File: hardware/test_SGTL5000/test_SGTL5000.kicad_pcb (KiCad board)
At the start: 2 copper layers, 68 x 68 mm, 70 parts, among them J201 SWD, J301 LINEIN_R, J302 LINEIN_L, J303 MIC, J304 LINEOUT_L, J305 LINEOUT_R, J401 USB_C_Receptacle_USB2.0, SW201 RST, U201 STM32G431KBT6, U301 SGTL5000XNLA3, U401 USBLC6-2SC6, U501 BU33SD5WG-TR, U502 BU33SD5WG-TR, U503 BU18SD2MG-MTR, Y201 16MHz

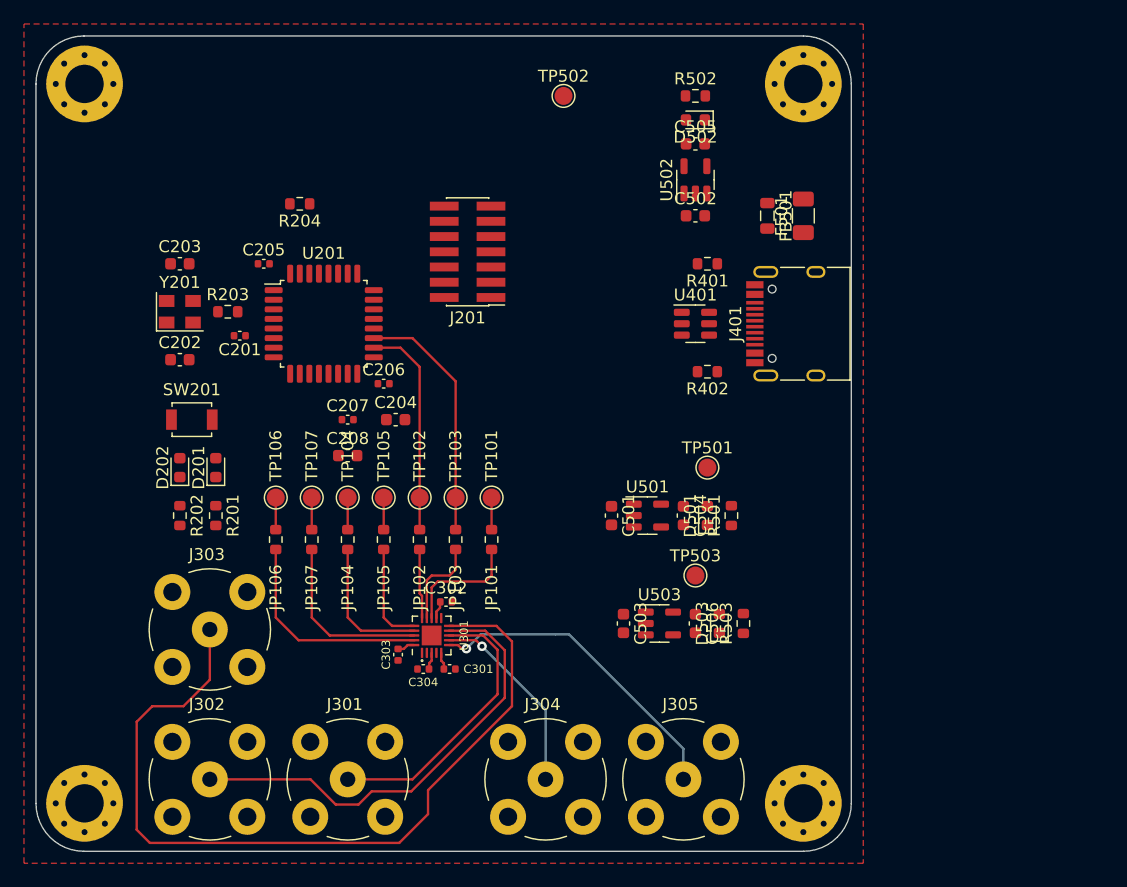
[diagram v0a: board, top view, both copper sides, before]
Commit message: Started routing
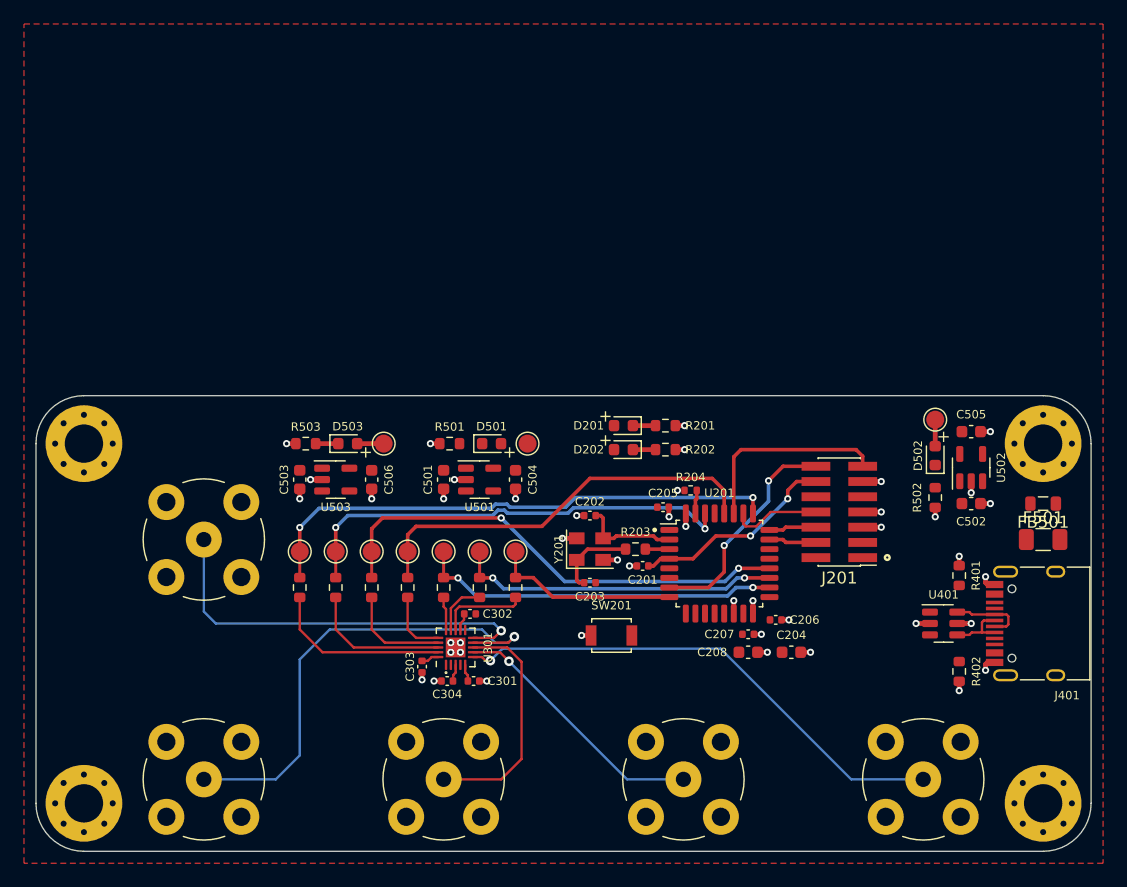
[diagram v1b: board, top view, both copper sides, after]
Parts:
- C202, C203: footprint Capacitor_SMD:C_0603_1608Metric -> Capacitor_SMD:C_0402_1005Metric
- R204: footprint Resistor_SMD:R_0603_1608Metric -> Resistor_SMD:R_0402_1005Metric
- moved C203 43.3 mm to (62.2, 61.6), turned to 180 degrees
- moved TP502 41.1 mm to (91.0, 48.0)
- moved R202 40.9 mm to (68.5, 50.5), turned to 0 degrees
- moved R204 40.4 mm to (70.6, 53.9)
- moved Y201 39.5 mm to (62.2, 58.8)
- moved R503 39.5 mm to (38.5, 50.0), turned to 180 degrees
- moved SW201 39.4 mm to (64.0, 66.0)
- moved R203 39.3 mm to (66.0, 58.8)
- moved R502 39.0 mm to (91.0, 54.5), turned to -90 degrees
- moved C205 39.0 mm to (68.3, 55.3)
- moved C201 38.7 mm to (66.6, 60.2)
- moved U201 38.6 mm to (73.0, 60.0)
- moved C204 38.3 mm to (79.0, 67.4)
- moved R201 38.2 mm to (68.5, 48.5), turned to 0 degrees
- moved C206 38.2 mm to (77.7, 64.7)
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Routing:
- net /STM32/I2C_SCL: track 2.67 -> 44.5 mm, vias 0 -> 2
- net /STM32/I2S_DIN: track 2.67 -> 40.3 mm, vias 0 -> 2
- net /CODEC/MIC: track 69.6 -> 34.1 mm, vias 0 -> 1
- net GND: track 0.00 -> 35.3 mm, vias 0 -> 43
- net /STM32/I2C_SDA: track 2.67 -> 37.9 mm, vias 0 -> 2
- net /STM32/I2S_DOUT: track 2.67 -> 34.3 mm
- net /STM32/VCP_TX: track 0.00 -> 18.7 mm, vias 0 -> 2
- net /STM32/nRST: track 0.00 -> 17.3 mm, vias 0 -> 2
- net /STM32/VCP_RX: track 0.00 -> 16.8 mm
- net /CODEC/LINEOUT_R: track 26.7 -> 42.6 mm
- net /STM32/SYS_MCLK: track 2.67 -> 15.7 mm
- net /STM32/I2S_SCLK: track 18.1 -> 30.3 mm, vias 0 -> 2
- net /STM32/OSC_IN: track 0.00 -> 8.13 mm
- net /STM32/SWO: track 0.00 -> 7.50 mm
- net /STM32/XTAL_OUT: track 0.00 -> 6.85 mm
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- added copper zone on In1.Cu, net GND
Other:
- board size 68 x 68 mm -> 88 x 38 mm
- copper layers 2 -> 4
- board text added: "+"
